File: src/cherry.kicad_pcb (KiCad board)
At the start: 2 copper layers, 51 x 21 mm, 4 parts

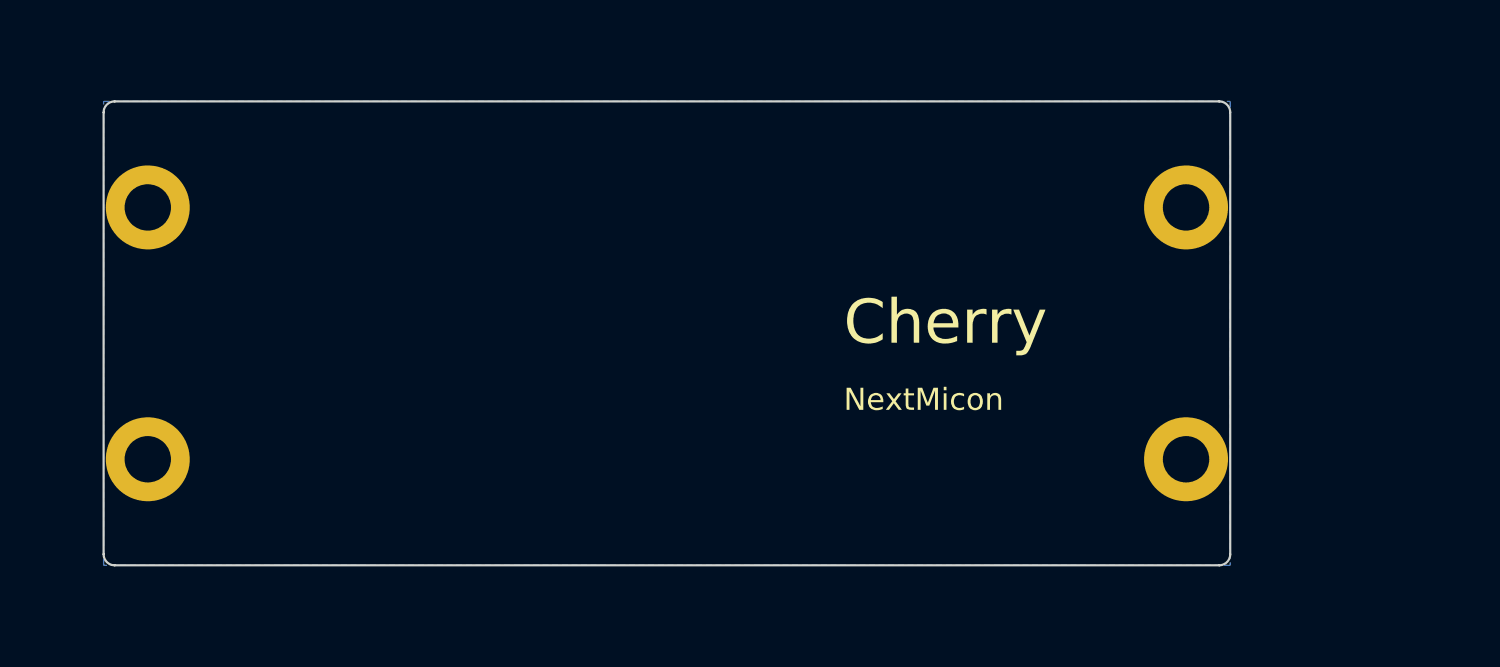
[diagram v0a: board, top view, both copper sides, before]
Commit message: wip: current layout state
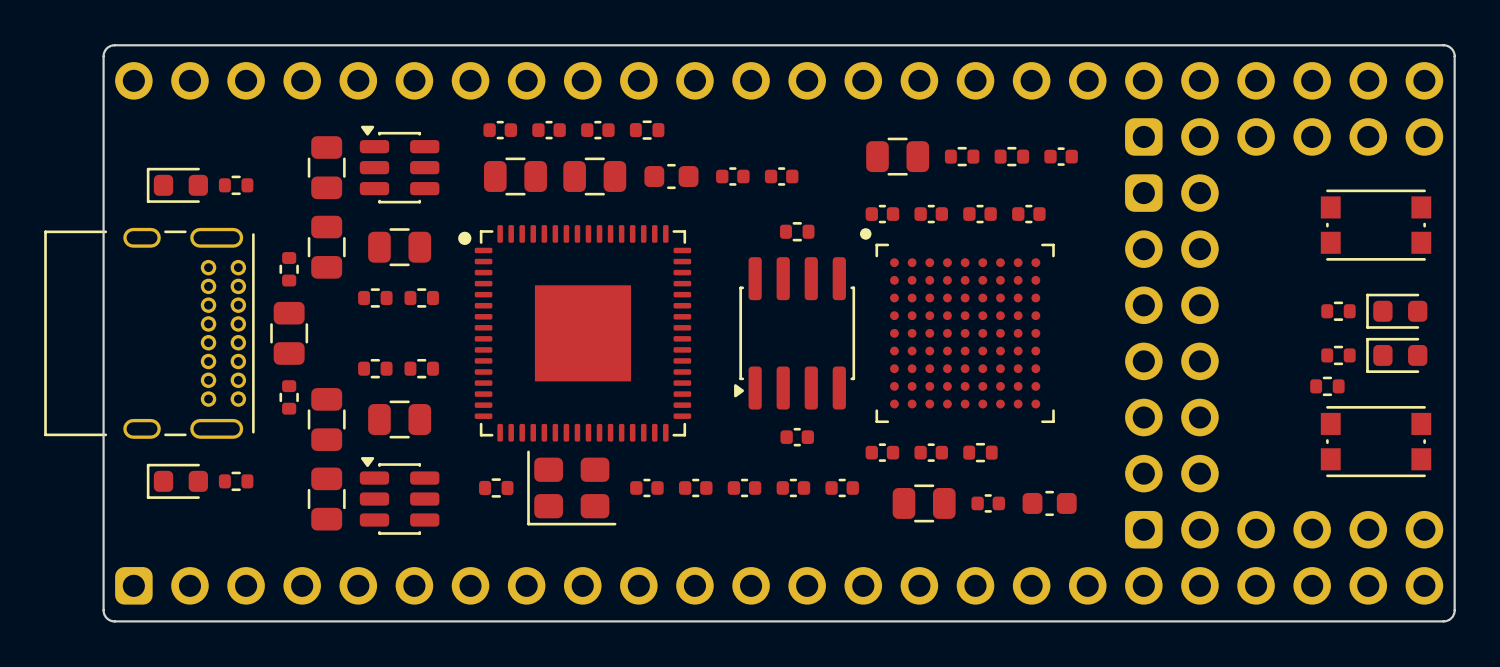
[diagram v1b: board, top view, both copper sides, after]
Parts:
- removed H1, H2, H3, H4: MountingHole, Cherry:MountingHole_2.1mm_M2
- added C1: 10uF, Cherry:C_0805_2012Metric, F.Cu at (110.1, 83.0)
- added C10: 100nF, Cherry:C_0402_1005Metric, F.Cu at (120.2, 81.3)
- added C11: 100nF, Cherry:C_0402_1005Metric, F.Cu at (122.4, 81.3)
- added C12: 100nF, Cherry:C_0402_1005Metric, F.Cu at (118.0, 81.3)
- added C13: 100nF, Cherry:C_0402_1005Metric, F.Cu at (128.5, 83.4)
- added C14: 100nF, Cherry:C_0402_1005Metric, F.Cu at (130.7, 83.4)
- added C15: 10uF, Cherry:C_0805_2012Metric, F.Cu at (118.6, 83.4)
- added C16: 100nF, Cherry:C_0402_1005Metric, F.Cu at (124.6, 97.5)
- added C17: 100nF, Cherry:C_0402_1005Metric, F.Cu at (135.3, 95.9)
- added C18: 100nF, Cherry:C_0402_1005Metric, F.Cu at (137.5, 95.9)
- added C19: 10uF, Cherry:C_0805_2012Metric, F.Cu at (137.1, 98.2)
- added C2: 10uF, Cherry:C_0805_2012Metric, F.Cu at (110.1, 98.0)
- added C20: 100nF, Cherry:C_0402_1005Metric, F.Cu at (135.3, 85.1)
- added C21: 100nF, Cherry:C_0402_1005Metric, F.Cu at (137.5, 85.1)
- added C22: 100nF, Cherry:C_0402_1005Metric, F.Cu at (139.7, 85.1)
- added C23: 100nF, Cherry:C_0402_1005Metric, F.Cu at (141.9, 85.1)
- added C24: 100nF, Cherry:C_0402_1005Metric, F.Cu at (143.3, 82.5)
- added C25: 10uF, Cherry:C_0805_2012Metric, F.Cu at (135.9, 82.5)
- added C26: 100nF, Cherry:C_0402_1005Metric, F.Cu at (140.0, 98.2)
- added C27: 10uF, Cherry:C_0603_1608Metric, F.Cu at (142.8, 98.2)
- added C28: 100nF, Cherry:C_0402_1005Metric, F.Cu at (131.4, 95.2)
- added C3: 22uF, Cherry:C_0805_2012Metric, F.Cu at (110.1, 86.6)
- added C4: 22uF, Cherry:C_0805_2012Metric, F.Cu at (110.1, 94.4)
- added C5: 4.7uF, Cherry:C_0603_1608Metric, F.Cu at (125.7, 83.4)
- added C6: 100nF, Cherry:C_0402_1005Metric, F.Cu at (126.8, 97.5)
- added C7: 100nF, Cherry:C_0402_1005Metric, F.Cu at (129.0, 97.5)
- added C8: 100nF, Cherry:C_0402_1005Metric, F.Cu at (131.2, 97.5)
- added C9: 100nF, Cherry:C_0402_1005Metric, F.Cu at (133.4, 97.5)
- added D1: PWR, Cherry:LED_0603_1608Metric, F.Cu at (103.5, 83.8)
- added D2: CFG, Cherry:LED_0603_1608Metric, F.Cu at (103.5, 97.2)
- added D3: USER0, Cherry:LED_0603_1608Metric, F.Cu at (158.7, 89.5)
- added D4: USER1, Cherry:LED_0603_1608Metric, F.Cu at (158.7, 91.5)
- added FB1: BLM21AG601SH1D, Cherry:L_0805_2012Metric, F.Cu at (108.4, 90.5)
- added FB2: BLM21AG601SH1D, Cherry:L_0805_2012Metric, F.Cu at (122.2, 83.4)
- added J1: USB4085-GF-A, Cherry:USB_C_Receptacle_GCT_USB4085, F.Cu at (106.1, 87.5)
- added J2: PinHeader_2x24, Cherry:PinHeader_2x24_P2.54mm_Rows22.86mm, F.Cu at (130.6, 90.5)
- added J3: PinHeader_2x06, Cherry:PinHeader_2x06_P2.54mm_Vertical, F.Cu at (148.4, 90.5)
- added J4: PinHeader_1x06, Cherry:PinHeader_1x06_P2.54mm, F.Cu at (153.4, 81.6)
- added J5: PinHeader_1x06, Cherry:PinHeader_1x06_P2.54mm, F.Cu at (153.4, 99.4)
- added L1: 1uH, Cherry:L_0805_2012Metric, F.Cu at (113.4, 86.6)
- added L2: 1uH, Cherry:L_0805_2012Metric, F.Cu at (113.4, 94.4)
- added R1: 180k, Cherry:R_0402_1005Metric, F.Cu at (112.3, 88.9)
- added R10: 10k, Cherry:R_0402_1005Metric, F.Cu at (138.9, 82.5)
- added R11: 10k, Cherry:R_0402_1005Metric, F.Cu at (131.4, 85.9)
- added R12: 10k, Cherry:R_0402_1005Metric, F.Cu at (155.4, 92.9)
- added R13: 100, Cherry:R_0402_1005Metric, F.Cu at (139.7, 95.9)
- added R14: 1k, Cherry:R_0402_1005Metric, F.Cu at (106.0, 83.8)
- added R15: 1k, Cherry:R_0402_1005Metric, F.Cu at (106.0, 97.2)
- added R16: 1k, Cherry:R_0402_1005Metric, F.Cu at (155.9, 89.5)
- added R17: 1k, Cherry:R_0402_1005Metric, F.Cu at (155.9, 91.5)
- added R2: 39.2k, Cherry:R_0402_1005Metric, F.Cu at (114.4, 88.9)
- added R3: 100k, Cherry:R_0402_1005Metric, F.Cu at (112.3, 92.1)
- added R4: 100k, Cherry:R_0402_1005Metric, F.Cu at (114.4, 92.1)
- added R5: 5.1k, Cherry:R_0402_1005Metric, F.Cu at (108.4, 87.6)
- added R6: 5.1k, Cherry:R_0402_1005Metric, F.Cu at (108.4, 93.4)
- added R7: 12k, Cherry:R_0402_1005Metric, F.Cu at (117.8, 97.5)
- added R8: 10k, Cherry:R_0402_1005Metric, F.Cu at (124.6, 81.3)
- added R9: 10k, Cherry:R_0402_1005Metric, F.Cu at (141.1, 82.5)
- added SW1: RESET, Cherry:SW_Push_1P1T_NO_CK_KMR2, F.Cu at (157.6, 85.6)
- added SW2: USER, Cherry:SW_Push_1P1T_NO_CK_KMR2, F.Cu at (157.6, 95.4)
- added U1: FT2232HQ, Cherry:QFN-64-1EP_9x9mm_P0.5mm_EP4.35x4.35mm, F.Cu at (121.7, 90.5)
- added U2: ICE40LP8K-CM81, Cherry:BGA-81_9x9_8.0x8.0mm_P0.8mm, F.Cu at (139.0, 90.5)
- added U3: W25Q32JVSSIQ, Cherry:SOIC-8_3.9x4.9mm_P1.27mm, F.Cu at (131.4, 90.5)
- added U4: TPS62A02, Cherry:SOT-23-6, F.Cu at (113.4, 83.0)
- added U5: TPS62A02, Cherry:SOT-23-6, F.Cu at (113.4, 98.0)
- added X1: ASE-12.000MHZ-LC-T, Cherry:Oscillator_SMD_Abracon_ASE-4Pin_3.2x2.5mm, F.Cu at (121.2, 97.5)
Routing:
- removed copper zone on B.Cu, net GND
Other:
- board size 51 x 21 mm -> 61.2 x 26.1 mm
